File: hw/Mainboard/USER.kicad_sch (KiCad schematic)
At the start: 1 part, among them J4 USER

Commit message: hw: wip add MCU, 2 layer board
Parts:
- J4: footprint PET:EDGE_CON_24P_USER -> Retrocomputing:CBM_PET_USER_EDGE_CON_24P; symbol Mainboard-rescue:Conn_02x12_Card_Edge-PET -> Retrocomputing:CBM_PET_USER_Conn_02x12_Card_Edge
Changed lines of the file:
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@@
     (effects (font (size 1.27 1.27)) (justify right))
   )
-  (symbol (lib_id "Mainboard-rescue:Conn_02x12_Card_Edge-PET") (at 133.35 69.85 0) (unit 1)
+  (symbol (lib_id "Retrocomputing:CBM_PET_USER_Conn_02x12_Card_Edge") (at 133.35 69.85 0) (unit 1)
     (in_bom yes) (on_board yes)
     (property "Reference" "J4" (id 0) (at 134.62 51.6382 0))
     (property "Value" "USER" (id 1) (at 134.62 53.9496 0))
-    (property "Footprint" "PET:EDGE_CON_24P_USER" (id 2) (at 133.35 69.85 0)
+    (property "Footprint" "Retrocomputing:CBM_PET_USER_EDGE_CON_24P" (id 2) (at 133.35 69.85 0)
       (effects (font (size 1.27 1.27)) hide)
     )

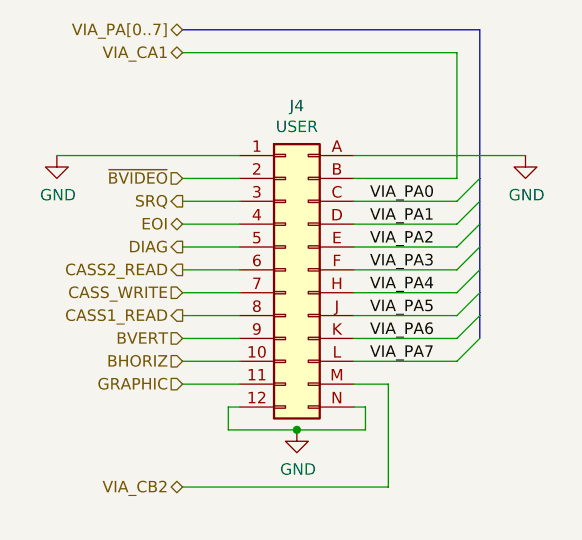
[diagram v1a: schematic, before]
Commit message: hw: routable (wip)
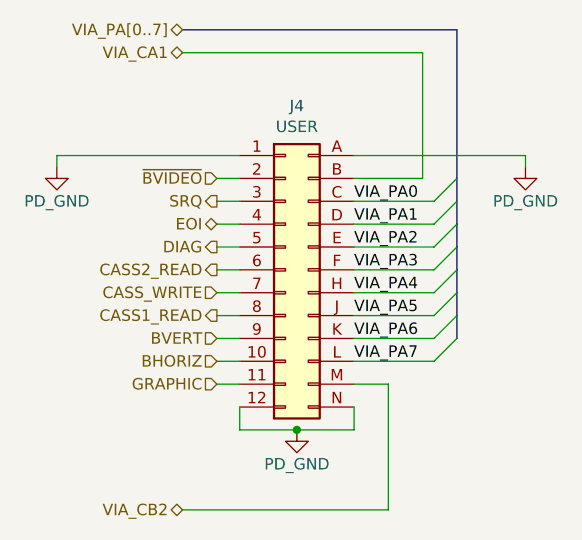
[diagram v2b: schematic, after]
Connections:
- net GND renamed PD_GND
